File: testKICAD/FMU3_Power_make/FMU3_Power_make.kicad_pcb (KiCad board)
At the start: 2 copper layers, 18 x 10.5 mm, 12 parts, among them J1 Conn_01x03_Male, J2 Conn_01x04_Female, U1 MIC5332-SSYMT-TR

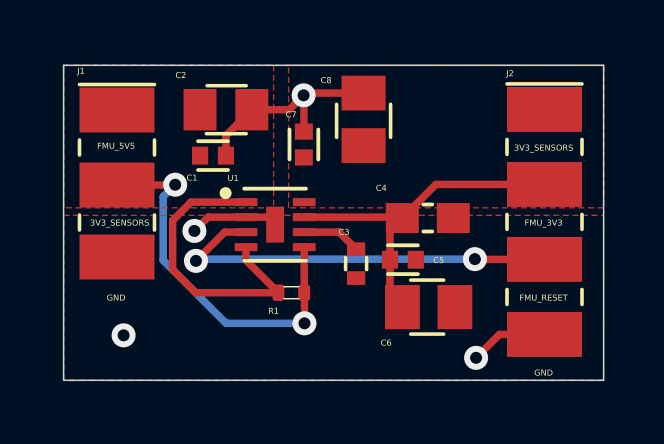
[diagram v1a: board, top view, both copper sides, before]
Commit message: save
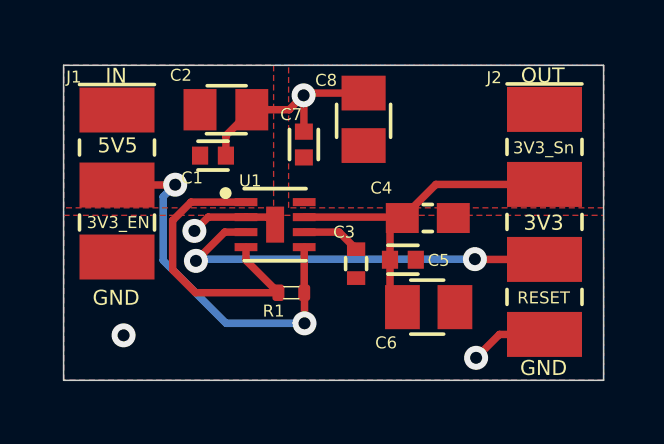
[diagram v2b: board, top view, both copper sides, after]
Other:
- board text added: "3V3"
- board text added: "3V3_EN"
- board text added: "3V3_Sn"
- board text added: "5V5"
- board text added: "IN"
- board text added: "OUT"
- board text added: "RESET"
- board text removed: "3V3_SENSORS"
- board text removed: "FMU_3V3"
- board text removed: "FMU_5V5"
- board text removed: "FMU_RESET"
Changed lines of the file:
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@@
-(kicad_pcb (version 20171130) (host pcbnew "(5.1.6)-1")
+(kicad_pcb (version 20171130) (host pcbnew "(5.1.5)-3")
   (general
     (thickness 1.6)
-    (drawings 11)
+    (drawings 13)
     (tracks 54)
     (zones 0)
@@
   (page A4)
   (layers
-    (0 F.Cu signal hide)
-    (31 B.Cu signal hide)
+    (0 F.Cu signal)
+    (31 B.Cu signal)
     (32 B.Adhes user hide)
     (33 F.Adhes user hide)
-    (34 B.Paste user hide)
-    (35 F.Paste user hide)
+    (34 B.Paste user)
+    (35 F.Paste user)
     (36 B.SilkS user)
     (37 F.SilkS user)
-    (38 B.Mask user)
-    (39 F.Mask user)
+    (38 B.Mask user hide)
+    (39 F.Mask user hide)
     (40 Dwgs.User user hide)
     (41 Cmts.User user hide)
@@
     (44 Edge.Cuts user)
     (45 Margin user hide)
-    (46 B.CrtYd user)
-    (47 F.CrtYd user)
+    (46 B.CrtYd user hide)
+    (47 F.CrtYd user hide)
     (48 B.Fab user hide)
     (49 F.Fab user hide)
@@
     (at 109.51 52.14 90)
     (fp_text reference C7 (at 1 -0.425 180) (layer F.SilkS)
-      (effects (font (size 0.2 0.2) (thickness 0.05)))
+      (effects (font (size 0.4 0.4) (thickness 0.05)))
     )
     (fp_text value 0u1 (at 0.3 0.75 90) (layer F.Fab)
@@
     (at 109.08 57.09 180)
     (fp_text reference R1 (at 0.58 -0.6) (layer F.SilkS)
-      (effects (font (size 0.2 0.2) (thickness 0.05)))
+      (effects (font (size 0.4 0.4) (thickness 0.05)))
     )
     (fp_text value 10K (at 0.75 0.625) (layer F.Fab)
@@
     (at 112.81 55.98)
     (fp_text reference C5 (at 1.19 0.02) (layer F.SilkS)
-      (effects (font (size 0.2 0.2) (thickness 0.05)))
+      (effects (font (size 0.4 0.4) (thickness 0.05)))
     )
     (fp_text value 0u1 (at 0.3 0.75) (layer F.Fab)
@@
   (module woos_FMU3:Conn_01x04_SMD (layer F.Cu)
     (at 115.98 49.87)
-    (fp_text reference J2 (at 0.4 -0.1) (layer F.SilkS)
-      (effects (font (size 0.2 0.2) (thickness 0.05)))
+    (fp_text reference J2 (at -0.13 0.04) (layer F.SilkS)
+      (effects (font (size 0.4 0.4) (thickness 0.05)))
     )
     (fp_text value Conn_01x04_Female (at 1.3 9.9) (layer F.Fab)
@@
     (at 106.48 52.51)
     (fp_text reference C1 (at -0.7 0.74) (layer F.SilkS)
-      (effects (font (size 0.2 0.2) (thickness 0.05)))
+      (effects (font (size 0.4 0.4) (thickness 0.05)))
     )
     (fp_text value 0u1 (at 0.3 0.75) (layer F.Fab)
@@
     (at 106.91 50.98)
     (fp_text reference C2 (at -1.5 -1.15) (layer F.SilkS)
-      (effects (font (size 0.2 0.2) (thickness 0.05)))
+      (effects (font (size 0.4 0.4) (thickness 0.05)))
     )
     (fp_text value 10u/25V (at -0.5 1.2) (layer F.Fab)
@@
     (at 111.25 56.11 270)
     (fp_text reference C3 (at -1.05 0.4 180) (layer F.SilkS)
-      (effects (font (size 0.2 0.2) (thickness 0.05)))
+      (effects (font (size 0.4 0.4) (thickness 0.05)))
     )
     (fp_text value CC0402KRX7R7BB103 (at 0.3 0.75 90) (layer F.Fab)
@@
     (descr <b>CAPACITOR</b>)
     (fp_text reference C4 (at -1.55 -1) (layer F.SilkS)
-      (effects (font (size 0.2 0.2) (thickness 0.05)))
+      (effects (font (size 0.4 0.4) (thickness 0.05)))
     )
     (fp_text value 1u (at -0.625 1.025) (layer F.Fab)
@@
     (at 113.67 57.56)
     (fp_text reference C6 (at -1.42 1.19) (layer F.SilkS)
-      (effects (font (size 0.2 0.2) (thickness 0.05)))
+      (effects (font (size 0.4 0.4) (thickness 0.05)))
     )
     (fp_text value 22u/25V (at -0.525 1.3) (layer F.Fab)
@@
     (at 111.5 51.3 90)
     (fp_text reference C8 (at 1.3 -1.25 180) (layer F.SilkS)
-      (effects (font (size 0.2 0.2) (thickness 0.05)))
+      (effects (font (size 0.4 0.4) (thickness 0.05)))
     )
     (fp_text value 22u/25V (at -0.525 1.3 90) (layer F.Fab)
@@
   (module woos_FMU3:Conn_01x03_SMD (layer F.Cu)
     (at 101.58 49.89)
-    (fp_text reference J1 (at 0.5 -0.2) (layer F.SilkS)
-      (effects (font (size 0.2 0.2) (thickness 0.05)))
+    (fp_text reference J1 (at 0.26 0) (layer F.SilkS)
+      (effects (font (size 0.4 0.4) (thickness 0.05)))
     )
     (fp_text value Conn_01x03_Male (at 1.4 7.3) (layer F.Fab)
@@
   (module MIC5332-SSYMT-TR:SON50P200X200X60-9N (layer F.Cu)
     (at 108.55 54.81)
-    (fp_text reference U1 (at -1.4 -1.55) (layer F.SilkS)
-      (effects (font (size 0.2 0.2) (thickness 0.05)))
+    (fp_text reference U1 (at -0.83 -1.46) (layer F.SilkS)
+      (effects (font (size 0.4 0.4) (thickness 0.05)))
     )
     (fp_text value MIC5332-SSYMT-TR (at 0.3 1.7) (layer F.Fab)
@@
     )
   )
-  (gr_text GND (at 117.5 59.75) (layer F.SilkS)
-    (effects (font (size 0.2 0.2) (thickness 0.05)))
+  (gr_text OUT (at 117.47 49.84) (layer F.SilkS)
+    (effects (font (size 0.5 0.5) (thickness 0.05)))
+  )
+  (gr_text IN (at 103.25 49.85) (layer F.SilkS)
+    (effects (font (size 0.5 0.5) (thickness 0.05)))
+  )
+  (gr_text GND (at 117.5 59.59) (layer F.SilkS)
+    (effects (font (size 0.5 0.5) (thickness 0.05)))
   )
   (gr_text GND (at 103.25 57.25) (layer F.SilkS)
-    (effects (font (size 0.2 0.2) (thickness 0.05)))
+    (effects (font (size 0.5 0.5) (thickness 0.05)))
   )
   (gr_line (start 119.5 49.5) (end 119.5 60) (layer Edge.Cuts) (width 0.05))
-  (gr_text 3V3_SENSORS (at 103.37 54.75) (layer F.SilkS)
-    (effects (font (size 0.2 0.2) (thickness 0.05)))
-  )
-  (gr_text "FMU_5V5\n" (at 103.25 52.19) (layer F.SilkS)
-    (effects (font (size 0.2 0.2) (thickness 0.05)))
-  )
-  (gr_text "FMU_RESET\n" (at 117.5 57.25) (layer F.SilkS)
-    (effects (font (size 0.2 0.2) (thickness 0.05)))
-  )
-  (gr_text "FMU_3V3\n" (at 117.5 54.75) (layer F.SilkS)
-    (effects (font (size 0.2 0.2) (thickness 0.05)))
-  )
-  (gr_text 3V3_SENSORS (at 117.5 52.25) (layer F.SilkS)
-    (effects (font (size 0.2 0.2) (thickness 0.05)))
+  (gr_text 3V3_EN (at 103.32 54.74) (layer F.SilkS)
+    (effects (font (size 0.4 0.4) (thickness 0.05)))
+  )
+  (gr_text "5V5\n" (at 103.3 52.17) (layer F.SilkS)
+    (effects (font (size 0.5 0.5) (thickness 0.05)))
+  )
+  (gr_text "RESET\n" (at 117.5 57.25) (layer F.SilkS)
+    (effects (font (size 0.4 0.4) (thickness 0.05)))
+  )
+  (gr_text "3V3\n" (at 117.5 54.75) (layer F.SilkS)
+    (effects (font (size 0.5 0.5) (thickness 0.05)))
+  )
+  (gr_text 3V3_Sn (at 117.5 52.25) (layer F.SilkS)
+    (effects (font (size 0.4 0.4) (thickness 0.05)))
   )
   (gr_line (start 101.5 60) (end 101.5 49.5) (layer Edge.Cuts) (width 0.05))
